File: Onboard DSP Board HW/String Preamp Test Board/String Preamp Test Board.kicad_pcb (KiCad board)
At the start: 2 copper layers, 85.9 x 24.5 mm, 51 parts, among them J1 Conn_01x07_Socket, J2 Conn_01x07_Socket, J3 Battery, J4 Output Jack, U1 TLV9004, U2 TLV9001IDCK, U3 TLV9001IDCK, U5 TP4054

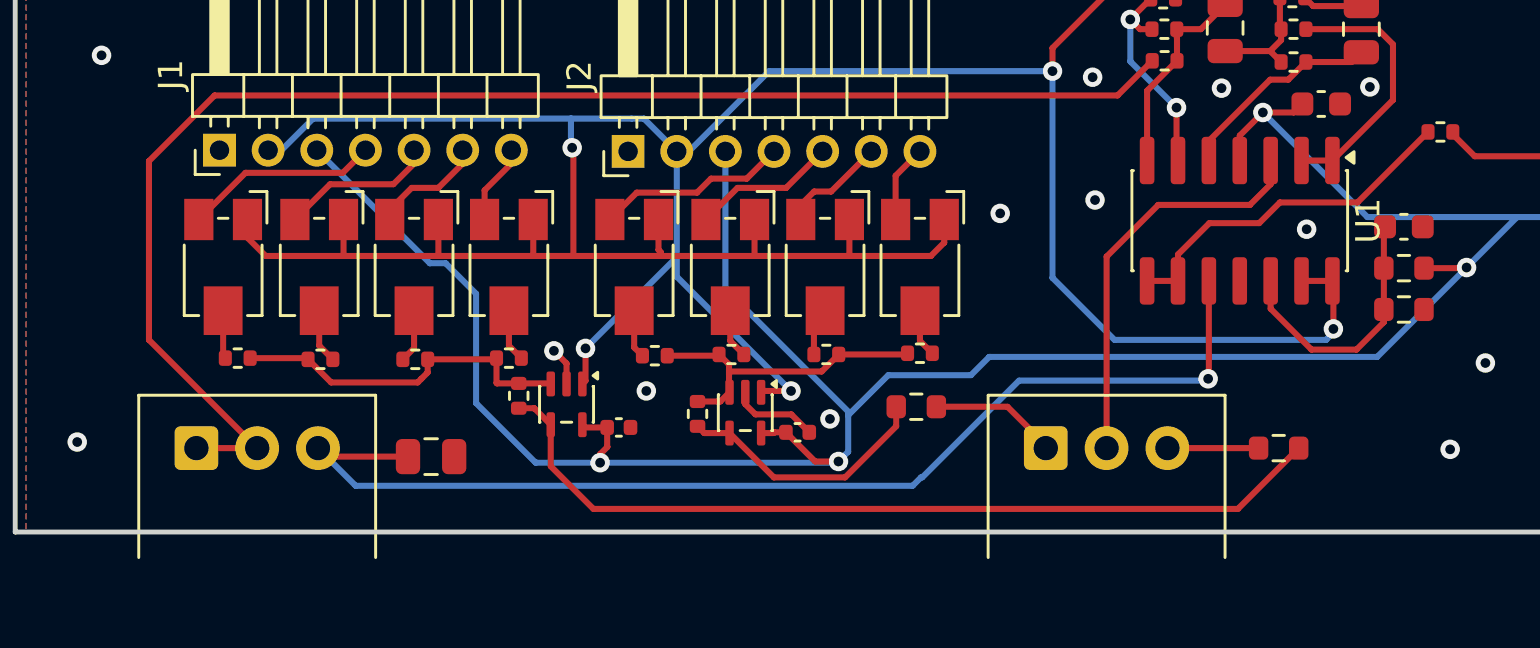
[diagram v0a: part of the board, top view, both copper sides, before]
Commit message: WIP
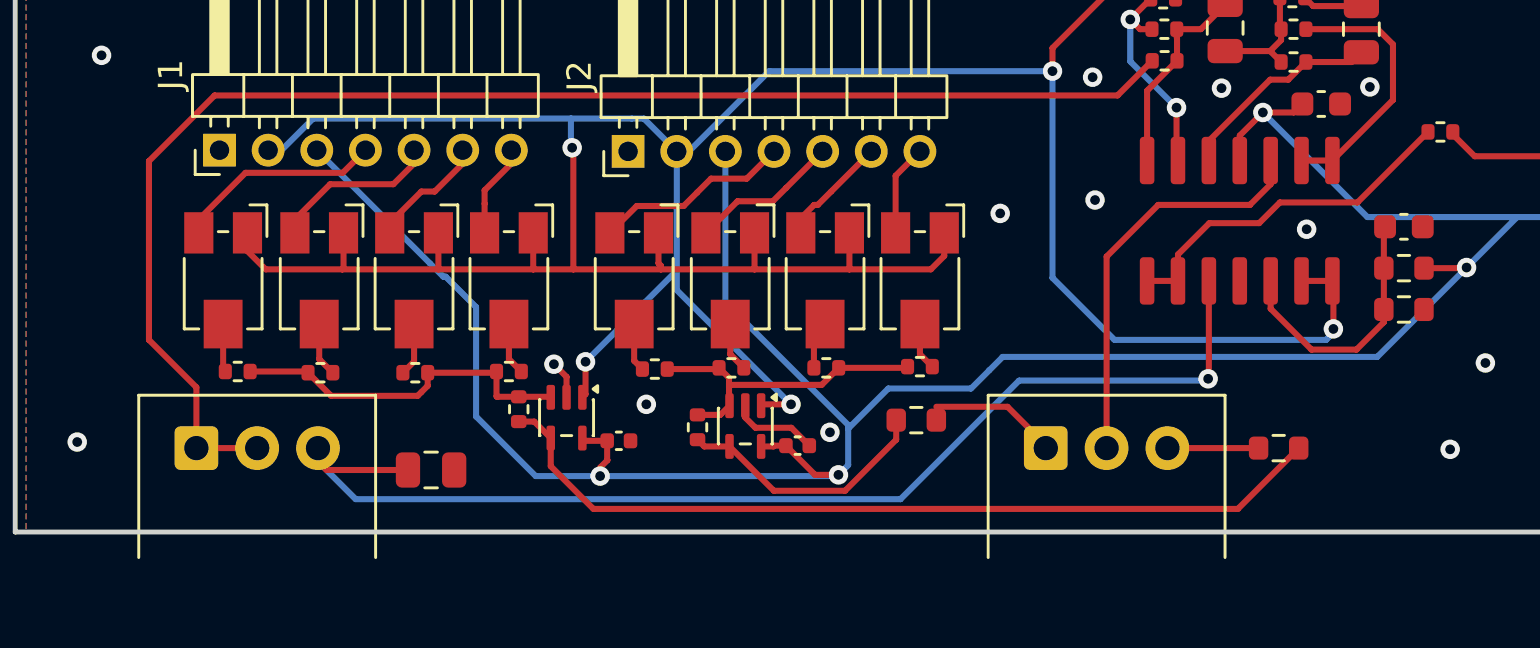
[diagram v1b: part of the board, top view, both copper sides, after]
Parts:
- moved C11 0.55 mm to (98.7, 77.4)
- moved C6 0.55 mm to (83.7, 78.4)
- moved R11 0.55 mm to (83.0, 74.4)
- moved R12 0.55 mm to (79.1, 74.4)
- moved R16 0.55 mm to (87.3, 75.9)
- moved R17 0.55 mm to (103.8, 74.2)
- moved C9 0.55 mm to (91.4, 77.2)
- moved R10 0.55 mm to (86.8, 74.3)
- moved R13 0.55 mm to (75.7, 74.3)
- moved R18 0.55 mm to (99.9, 74.2)
- moved R19 0.55 mm to (96.0, 74.2)
- moved R2 0.55 mm to (103.6, 76.3)
- moved R20 0.55 mm to (92.8, 74.2)
- moved R23 0.55 mm to (94.6, 76.6)
- moved RV10 0.55 mm to (96.0, 70.7)
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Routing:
- net /VG: track 141.1 -> 142.2 mm
- net /filt_out: track 59.1 -> 58.1 mm
- net /v+: track 121.2 -> 122.3 mm
- net Net-(J1-Pin_7): track 3.56 -> 4.11 mm
- net /p1_out: track 35.8 -> 35.3 mm
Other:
- rule pad_to_mask_clearance: 0 -> 0.05
